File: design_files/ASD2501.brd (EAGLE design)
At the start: 22.5 x 30.5 mm, 24 parts, among them J1 DF12-32-DP, J2 DF12-32-DS, U1 XC6210B18, U2 JF2, U3 TXS0102, U4 TXS0102

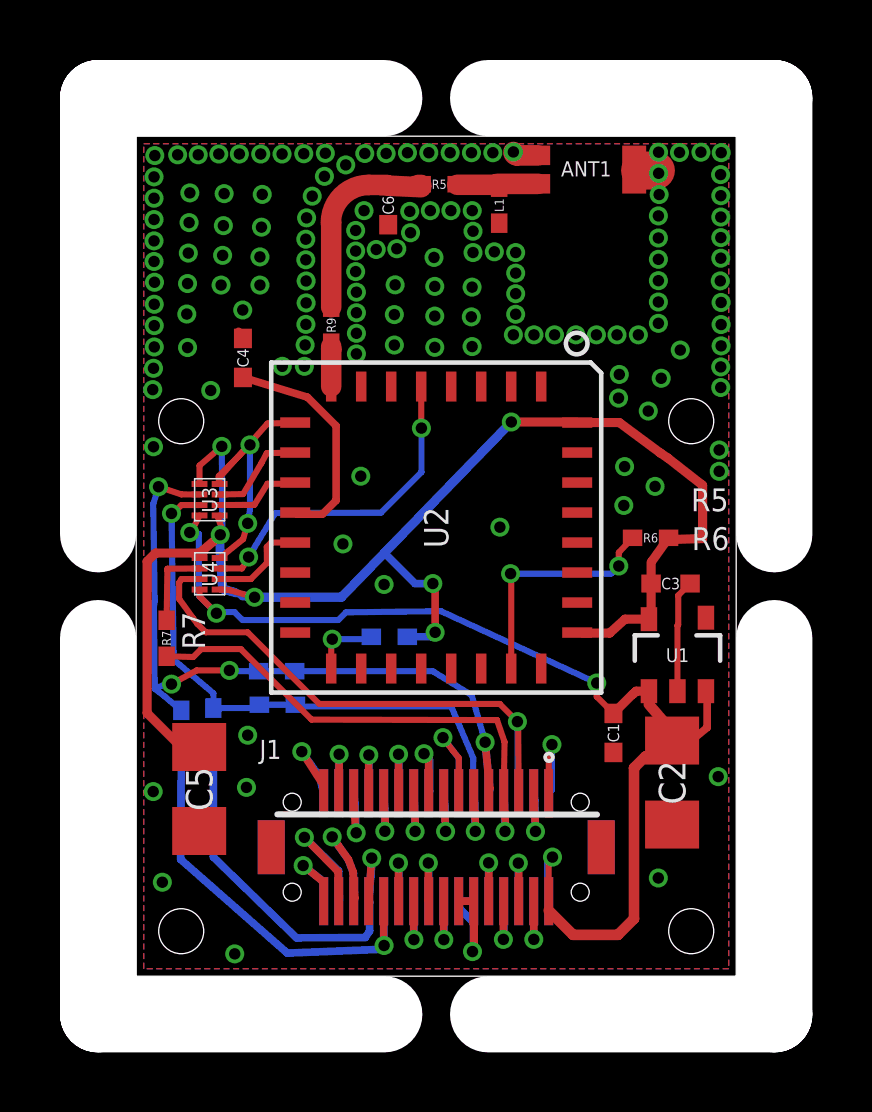
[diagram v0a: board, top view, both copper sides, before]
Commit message: update format
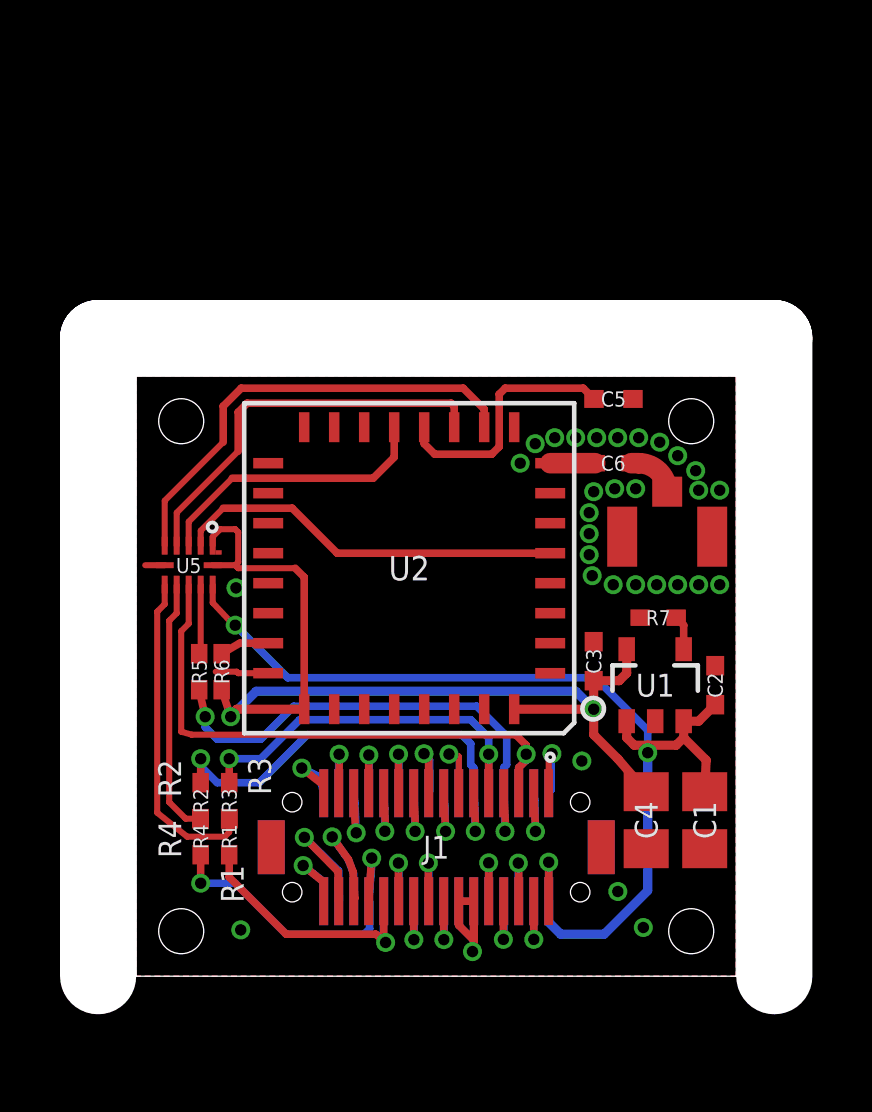
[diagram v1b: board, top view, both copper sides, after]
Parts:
- removed ANT1: AS-ITM-00109, tinycircuits:W3011
- removed L1: 1nH, tinycircuits:0402
- removed R8: 10.0K, tinycircuits:0402
- removed R9: 0.0, tinycircuits:0402
- removed U3, U4: TXS0102, tinycircuits:DQE(R-PX2SON-N8)
- added J3: U.FL-R-SMT(10), tinycircuits:U.FL-R-SMT(10)
- added U5: TXB0104, tinycircuits:UQFN-12
- C1, C4: value 0.1uF -> 10uF; device tinycircuits:C0402 -> tinycircuits:C0805
- C2, C5: value 47uF -> 0.1uF; device tinycircuits:C1206 -> tinycircuits:C0402
- C6: value 0.5pF -> 100pF; device tinycircuits:C0402 -> tinycircuits:0402
- R2, R3: device tinycircuits:0402_SHORT -> tinycircuits:0402
- moved C4 20.4 mm to (27.0, 15.2), turned to 270 degrees
- moved C5 19.0 mm to (25.9, 29.2), turned to 0 degrees
- moved R5 18.1 mm to (12.1, 20.1), turned to 270 degrees
- moved R7 16.4 mm to (27.4, 21.9), turned to 0 degrees
- moved R6 15.0 mm to (12.8, 20.1), turned to 270 degrees
- moved C6 11.4 mm to (25.9, 27.1), turned to 180 degrees
- moved R3 4.60 mm to (13.1, 15.8), flipped to the top, turned to 90 degrees
- moved C1 4.21 mm to (28.9, 15.2)
- moved R2 4.10 mm to (12.2, 15.8), flipped to the top, turned to 90 degrees
- moved R1 3.95 mm to (13.1, 14.7), flipped to the top
- moved R4 3.71 mm to (12.2, 14.7), flipped to the top
- moved C3 3.64 mm to (25.2, 20.5), turned to 90 degrees
- moved C2 3.55 mm to (29.3, 19.7), turned to 90 degrees
- moved U2 1.63 mm to (19.1, 23.6), turned to 180 degrees
- moved U1 1.25 mm to (27.3, 19.7)
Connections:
- removed net N$5 (its old number): ANT1.1, L1.1, R5.1
- new net N$14: U2.24
- new net N$6: R7.2, U1.4
- net AD2: now also R5.2; no longer R7.2
- net AD3: now also U5.9; no longer U4.7
- net GND: now also J3.GND1, J3.GND2, R7.1, U2.6, U5.6; no longer ANT1.2, ANT1.3, C6.2, L1.2, U3.4, U4.4
- net N$1: now also J3.ANT; no longer R5.2, R9.1
- net N$10: no longer R8.2
- net N$11: now also U5.3; no longer U4.2
- net N$12: now also U5.2; no longer U4.3
- net N$13: now also R5.1, U5.10; no longer R7.1, U4.6
- net N$2: now also U5.8; no longer U3.7
- net N$3: now also U5.7; no longer U3.6
- net N$4: now also U5.4; no longer U3.2
- net N$7: now also U5.5; no longer U3.3
- net N$8: now also C5.1; no longer C4.1
- net N$9: now also C6.2; no longer R9.2
- net VCC: now also U5.11; no longer U3.8, U4.8
- net VCC_1V8: now also C4.1, U5.1, U5.12; no longer C5.1, R8.1, U3.1, U3.5, U4.1, U4.5
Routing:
- net VCC_1V8: track 53.3 -> 35.3 mm, vias 6 -> 2
- net GND: track 21.7 -> 9.01 mm, vias 143 -> 31
- net N$7: track 3.31 -> 15.3 mm
- net N$4: track 2.93 -> 13.4 mm
- net N$5: track 8.01 -> 1.64 mm, vias 2 -> 0
- net N$11: track 3.34 -> 9.54 mm
- net N$1: track 6.71 -> 1.59 mm
- net IO0: track 15.1 -> 10.1 mm
- net AD0: track 10.8 -> 15.4 mm, vias 1 -> 2
- net VCC: track 39.7 -> 36.5 mm, vias 4 -> 3
- net IO1: track 15.3 -> 12.4 mm, vias 1 -> 2
- net N$5 (its old number): track 2.87 -> 0.00 mm
- net N$10: track 2.40 -> 0.00 mm, vias 1 -> 0
- net AD1: track 11.2 -> 13.4 mm, vias 1 -> 2
- net N$3: track 12.9 -> 10.9 mm, vias 3 -> 0
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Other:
- board size 22.5 x 30.5 mm -> 22.5 x 21.3 mm
- board text added: "4"
- board text added: "ASD2501 - Rev4"
- board text added: "TinyCircuits.com"
- board text added: "^ V-SCORE EDGE ALONG OUTLINE ^"
- board text removed: "3"
- board text removed: "ASD2501 - Rev3"
- board text removed: "R5"
- board text removed: "R6"
- board text removed: "R7"
- board text removed: "R8"
- board text removed: "Tiny-Circuits.com"
